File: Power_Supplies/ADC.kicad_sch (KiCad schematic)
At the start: 72 parts, among them IC1 PCM1808PWRG4, IC2 PCM1808PWRG4, IC3 PCM1808PWRG4, IC4 PCM1808PWRG4, IC5 PCM1808PWRG4, IC6 PCM1808PWRG4, IC7 PCM1808PWRG4, IC8 PCM1808PWRG4

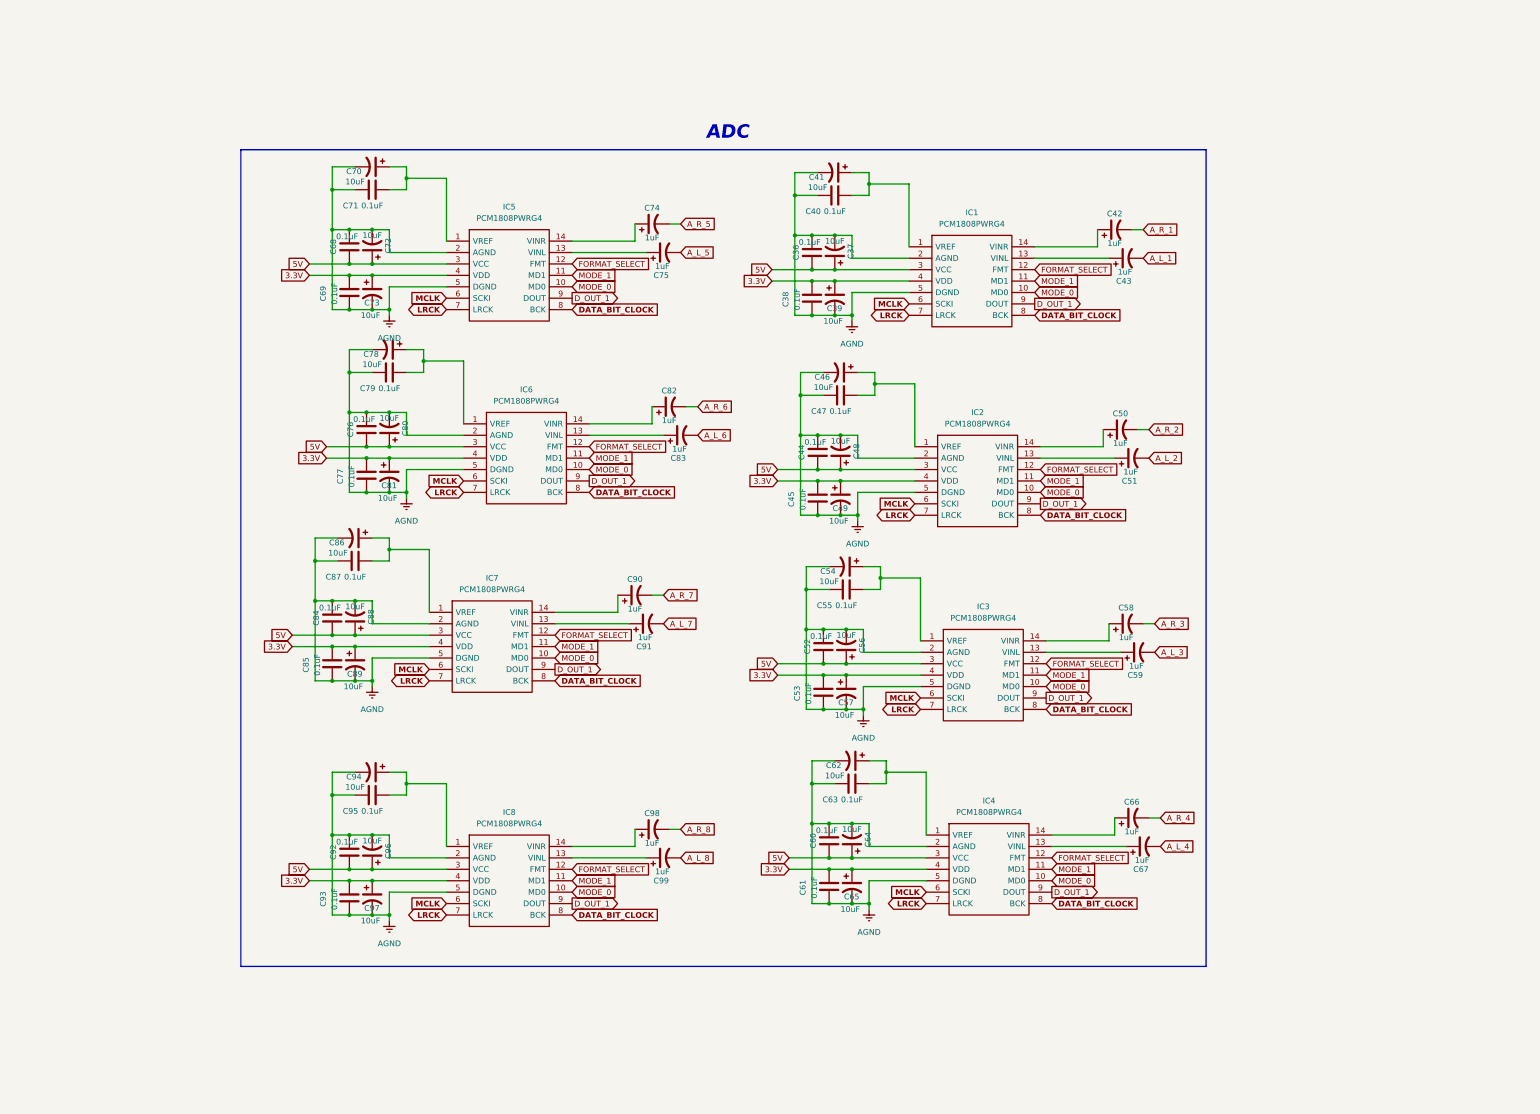
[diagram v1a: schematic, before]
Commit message: Add files via upload
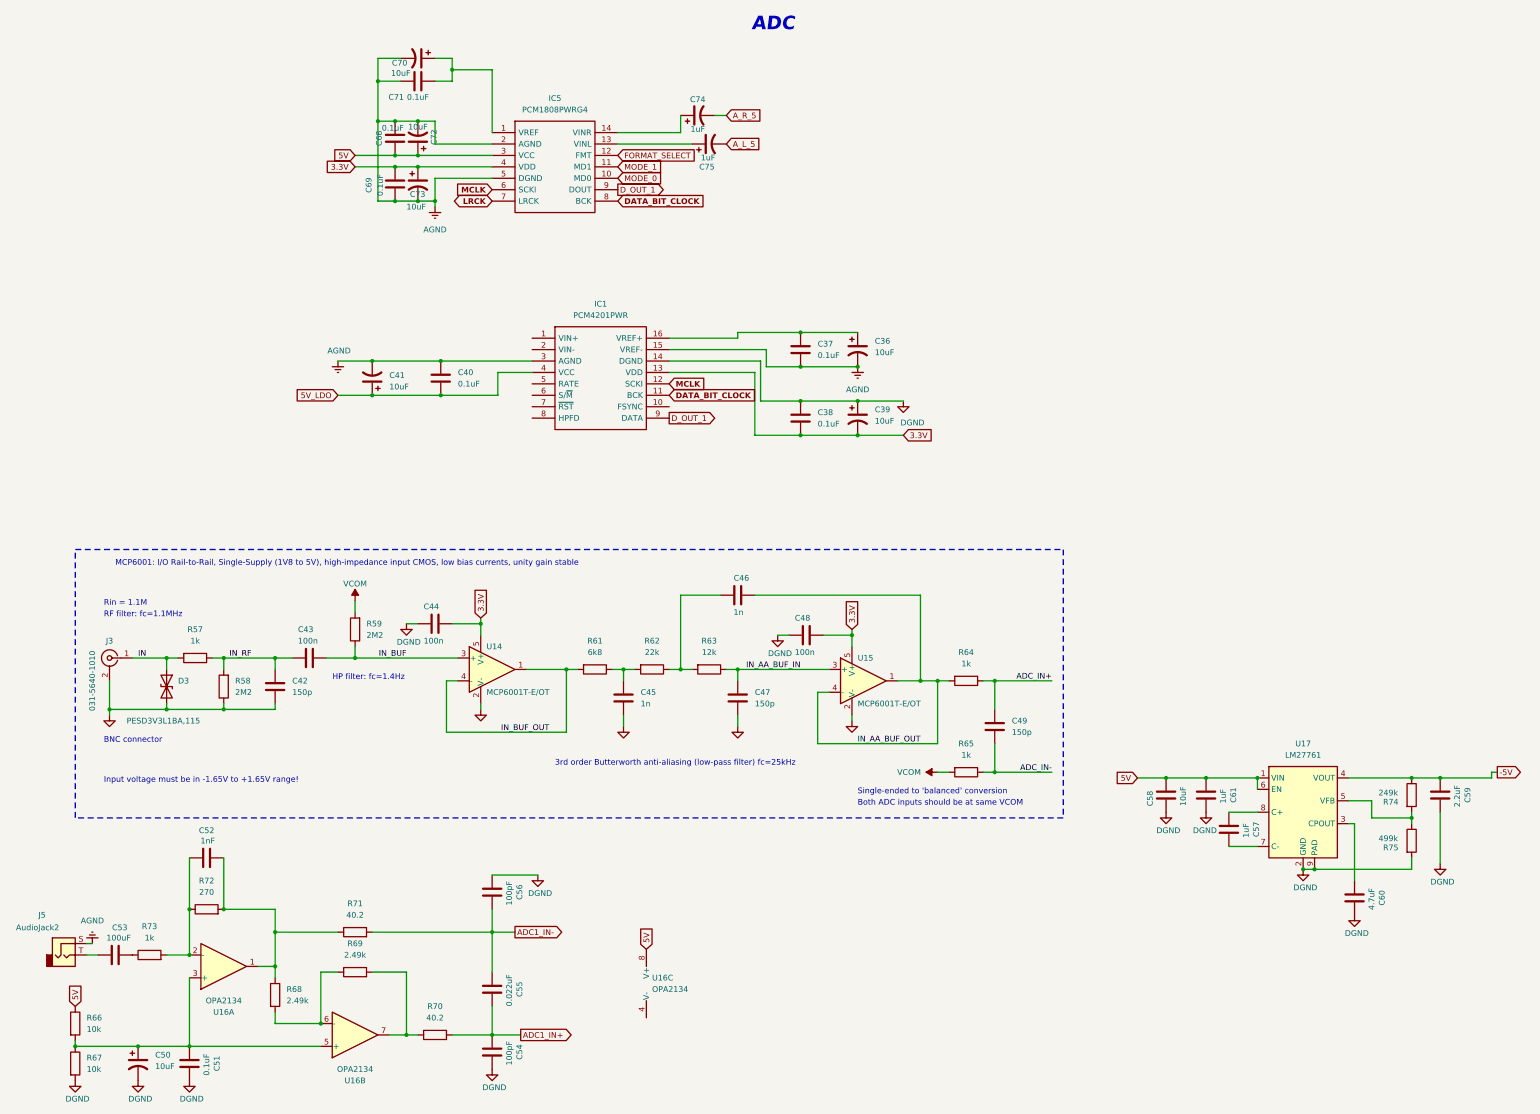
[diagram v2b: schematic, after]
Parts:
- removed C36, C63, C76, C77, C79, C84, C85, C87, C92, C93, C95: 0.1uF, Capacitor_SMD:C_0805_2012Metric, symbol Device:C
- removed C37, C46, C48, C49, C54, C56, C57, C62, C64, C65, C78, C80, C81, C86, C88, C89, C94, C96, C97: 10uF, Capacitor_SMD:CP_Elec_4x5.8, symbol Device:C_Polarized_US
- removed C42, C43, C51, C58, C59, C66, C67, C82, C83, C90, C91, C98, C99: 1uF, Capacitor_SMD:CP_Elec_4x5.8, symbol Device:C_Polarized_US
- removed IC1, IC2, IC3, IC4, IC6, IC7, IC8: PCM1808PWRG4, SamacSys_Parts:SOP65P640X120-14N, symbol SamacSys_Parts:PCM1808PWRG4
- added C36: 10uF, Capacitor_SMD:CP_Elec_4x5.8, symbol Device:C_Polarized_US
- added C37, C51: 0.1uF, Capacitor_SMD:C_0805_2012Metric, symbol Device:C
- added C42, C49: 150p, Capacitor_SMD:C_0402_1005Metric, symbol Device:C
- added C43, C48: 100n, Capacitor_SMD:C_0402_1005Metric, symbol Device:C
- added C46: 1n, Capacitor_SMD:C_0402_1005Metric, symbol Device:C
- added C54, C56: 100pF, Capacitor_SMD:C_0805_2012Metric, symbol Device:C
- added C57: 1uF, Capacitor_SMD:C_0805_2012Metric, symbol Device:C
- added C58: 10uF, Capacitor_SMD:C_0805_2012Metric, symbol Device:C
- added C59: 2.2uF, Capacitor_SMD:C_0805_2012Metric, symbol Device:C
- added D3: PESD3V3L1BA,115, Diode_SMD:D_SOD-323, symbol Device:D_TVS
- added IC1: PCM4201PWR, SOP65P640X120-16N, symbol SamacSys_Parts:PCM4201PWR
- added J3: 031-5640-1010, PhilsLab_Footprints_KiCad6:AMPHENOL-BNC-031-5640-1010, symbol Connector:Conn_Coaxial
- added J5: AudioJack2, symbol Connector_Audio:AudioJack2
- added R57, R64, R65: 1k, Resistor_SMD:R_0402_1005Metric, symbol Device:R
- added R58, R59: 2M2, Resistor_SMD:R_0402_1005Metric, symbol Device:R
- added R61: 6k8, Resistor_SMD:R_0402_1005Metric, symbol Device:R
- added R62: 22k, Resistor_SMD:R_0402_1005Metric, symbol Device:R
- added R63: 12k, Resistor_SMD:R_0402_1005Metric, symbol Device:R
- added R66, R67: 10k, Resistor_SMD:R_0805_2012Metric, symbol Device:R
- added R68, R69: 2.49k, Resistor_SMD:R_0805_2012Metric, symbol Device:R
- added R70, R71: 40.2, Resistor_SMD:R_0805_2012Metric, symbol Device:R
- added R72: 270, Resistor_SMD:R_0805_2012Metric, symbol Device:R
- added R73: 1k, Resistor_SMD:R_0805_2012Metric, symbol Device:R
- added R74: 249k, Resistor_SMD:R_0603_1608Metric, symbol Device:R
- added R75: 499k, Resistor_SMD:R_0603_1608Metric, symbol Device:R
- added U14, U15: MCP6001T-E/OT, Package_TO_SOT_SMD:SOT-23-5, symbol Amplifier_Operational:MCP6001-OT
- added U16: OPA2134, symbol Amplifier_Operational:OPA2134
- added U17: LM27761, Package_SON:WSON-8-1EP_2x2mm_P0.5mm_EP0.9x1.6mm, symbol Regulator_SwitchedCapacitor:LM27761
- C44: value 0.1uF -> 100n; footprint Capacitor_SMD:C_0805_2012Metric -> Capacitor_SMD:C_0402_1005Metric
- C45: value 0.1uF -> 1n; footprint Capacitor_SMD:C_0805_2012Metric -> Capacitor_SMD:C_0402_1005Metric
- C47: value 0.1uF -> 150p; footprint Capacitor_SMD:C_0805_2012Metric -> Capacitor_SMD:C_0402_1005Metric
- C50: value 1uF -> 10uF
- C52: value 0.1uF -> 1nF; footprint Capacitor_SMD:C_0805_2012Metric -> Capacitor_SMD:C_0402_1005Metric
- C53: value 0.1uF -> 100uF
- C55: value 0.1uF -> 0.022uF
- C60: value 0.1uF -> 4.7uF
- C61: value 0.1uF -> 1uF
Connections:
- net 3.3V: now also C39.2, C44.1, C48.1, IC1.13 (VDD), U14.5 (V+), U15.5 (V+); no longer C39.1, C45.2, C53.2, C61.2
- net 5V: now also C61.2, C58.2, R66.1, U16.8 (V+), U17.1 (VIN), U17.6 (EN); no longer C44.1, C52.1, C60.1
- net AGND: now also C40.1, C36.2, C37.2, IC1.15 (VREF-), IC1.3 (AGND), J5.S; no longer C38.1, C39.2, C40.2, C44.2, C45.1, C47.2, C52.2, C53.1, C55.2, C60.2, C61.1
- net DATA_BIT_CLOCK: now also IC1.11 (BCK)
- net D_OUT_1: now also IC1.9 (DATA)
- net MCLK: now also IC1.12 (SCKI)
- net ADC1_IN+: now reaches C55.1
- net ADC1_IN+: now also C54.2, R70.2
- net 5V_LDO: now reaches C41.1
- net 5V_LDO: now also C40.2, IC1.4 (VCC); no longer C40.1
- net IN_AA_BUF_IN: now reaches C47.1
- net IN_AA_BUF_IN: now also R63.1, U15.3 (+)
- net at C50.1: now also C51.2, R66.2, R67.1, U16.3 (+), U16.5 (+)
- net A_R_2 renamed DGND
- net DGND: now also C38.1, C39.1, C44.2, C60.1, C61.1, C48.2, C51.1, C54.1, C56.2, C58.1, C59.1, IC1.14 (DGND), R67.2, R75.2, U17.2 (GND), U17.9 (PAD)
- new net: C52.1, R68.1, R71.1, R72.2, U16.1
- new net: C52.2, R72.1, R73.2, U16.2 (-)
- new net: C46.1, R62.1, R63.2
- new net: C45.1, R61.1, R62.2
- new net: R68.2, R69.1, U16.6 (-)
- new net: C53.1, R73.1
- new net: C53.2, J5.T
- new net: R69.2, R70.1, U16.7
- new net: C36.1, C37.1, IC1.16 (VREF+)
- new net: R74.2, R75.1, U17.5 (VFB)
- new net: C60.2, U17.3 (CPOUT)
- new net: C57.1, U17.7 (C-)
- new net: C57.2, U17.8 (C+)
- new net -5V: C59.2, R74.1, U17.4 (VOUT)
- new net ADC1_IN-: C55.2, C56.1, R71.2
- new net ADC_IN+: C49.1, R64.1
- new net ADC_IN-: C49.2, R65.1
- new net GND: C42.2, C45.2, C47.2, D3.2 (A2), J3.2 (Ext), R58.1, U14.2 (V-), U15.2 (V-)
- new net IN: D3.1 (A1), J3.1 (In), R57.2
- new net IN_AA_BUF_OUT: C46.2, R64.2, U15.1, U15.4 (-)
- new net IN_BUF: C43.1, R59.1, U14.3 (+)
- new net IN_BUF_OUT: R61.2, U14.1, U14.4 (-)
- new net IN_RF: C42.1, C43.2, R57.1, R58.2
- new net VCOM: R59.2, R65.2
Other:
- note added: "3rd order Butterworth anti-aliasing (low-pass filter) fc=25kHz"
- note added: "BNC connector"
- note added: "Both ADC inputs should be at same VCOM"
- note added: "HP filter: fc=1.4Hz"
- note added: "Input voltage must be in -1.65V to +1.65V range!"
- note added: "MCP6001: I/O Rail-to-Rail, Single-Supply (1V8 to 5V), high-impedance input CMOS, low bias currents, unity gain stable"
- note added: "RF filter: fc=1.1MHz"
- note added: "Rin = 1.1M"
- note added: "Single-ended to 'balanced' conversion"
- moved on the sheet: C68, C69, C70, C71, C72, C73, C74, C75, IC5

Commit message: Add files via upload
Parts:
- removed C42, C47, C49: 150p, Capacitor_SMD:C_0402_1005Metric, symbol Device:C
- removed C43, C44, C48: 100n, Capacitor_SMD:C_0402_1005Metric, symbol Device:C
- removed C45, C46: 1n, Capacitor_SMD:C_0402_1005Metric, symbol Device:C
- removed C50, C70, C72, C73: 10uF, Capacitor_SMD:CP_Elec_4x5.8, symbol Device:C_Polarized_US
- removed C51, C68: 0.1uF, Capacitor_SMD:C_0805_2012Metric, symbol Device:C
- removed C74: 1uF, Capacitor_SMD:CP_Elec_4x5.8, symbol Device:C_Polarized_US
- removed D3: PESD3V3L1BA,115, Diode_SMD:D_SOD-323, symbol Device:D_TVS
- removed IC5: PCM1808PWRG4, SamacSys_Parts:SOP65P640X120-14N, symbol SamacSys_Parts:PCM1808PWRG4
- removed J3: 031-5640-1010, PhilsLab_Footprints_KiCad6:AMPHENOL-BNC-031-5640-1010, symbol Connector:Conn_Coaxial
- removed U14, U15: MCP6001T-E/OT, Package_TO_SOT_SMD:SOT-23-5, symbol Amplifier_Operational:MCP6001-OT
- added C121, C122, C123, C124, C70, C77, C84: 1nF, Capacitor_SMD:C_0402_1005Metric, symbol Device:C
- added C125, C127, C128, C130, C131, C133, C134, C136, C73, C78, C80, C85, C87: 100pF, Capacitor_SMD:C_0805_2012Metric, symbol Device:C
- added C126, C129, C132, C135, C72, C79, C86: 0.022uF, Capacitor_SMD:C_0805_2012Metric, symbol Device:C
- added C50, C67, C74, C81, C88, C89, C90, C91: 100uF, Capacitor_SMD:C_0805_2012Metric, symbol Device:C
- added C51, C68, C82, C92, C93, C94, C95: 10uF, Capacitor_SMD:CP_Elec_4x5.8, symbol Device:C_Polarized_US
- added C62: 10uF, Capacitor_SMD:C_0805_2012Metric, symbol Device:C
- added C63, C64: 1uF, Capacitor_SMD:C_0805_2012Metric, symbol Device:C
- added C65: 4.7uF, Capacitor_SMD:C_0805_2012Metric, symbol Device:C
- added C66: 2.2uF, Capacitor_SMD:C_0805_2012Metric, symbol Device:C
- added C76, C83, C96, C97, C98, C99: 0.1uF, Capacitor_SMD:C_0805_2012Metric, symbol Device:C
- added J10, J11, J12, J13, J3, J7, J9: AudioJack2, symbol Connector_Audio:AudioJack2
- added R100, R101, R78, R79, R86, R87, R94, R95, R96, R97, R98, R99: 10k, Resistor_SMD:R_0805_2012Metric, symbol Device:R
- added R102, R103, R104, R105, R80, R88: 1k, Resistor_SMD:R_0805_2012Metric, symbol Device:R
- added R106, R107, R108, R109, R81, R89: 270, Resistor_SMD:R_0805_2012Metric, symbol Device:R
- added R110, R111, R112, R113, R115, R117, R119, R121, R82, R84, R90, R92: 2.49k, Resistor_SMD:R_0805_2012Metric, symbol Device:R
- added R114, R116, R118, R120, R122, R123, R124, R125, R83, R85, R91, R93: 40.2, Resistor_SMD:R_0805_2012Metric, symbol Device:R
- added R76: 249k, Resistor_SMD:R_0603_1608Metric, symbol Device:R
- added R77: 499k, Resistor_SMD:R_0603_1608Metric, symbol Device:R
- added U14, U15, U19, U20, U21, U22, U23: OPA2134, symbol Amplifier_Operational:OPA2134
- added U18: LM27761, Package_SON:WSON-8-1EP_2x2mm_P0.5mm_EP0.9x1.6mm, symbol Regulator_SwitchedCapacitor:LM27761
- C52: value 1nF -> 0.1uF; footprint Capacitor_SMD:C_0402_1005Metric -> Capacitor_SMD:C_0805_2012Metric
- C53: value 100uF -> 1nF; footprint Capacitor_SMD:C_0805_2012Metric -> Capacitor_SMD:C_0402_1005Metric
- C71: value 0.1uF -> 100pF
- C75: value 1uF -> 10uF
- R57: value 1k -> 10k; footprint Resistor_SMD:R_0402_1005Metric -> Resistor_SMD:R_0805_2012Metric
- R58: value 2M2 -> 10k; footprint Resistor_SMD:R_0402_1005Metric -> Resistor_SMD:R_0805_2012Metric
- R59: value 2M2 -> 1k; footprint Resistor_SMD:R_0402_1005Metric -> Resistor_SMD:R_0805_2012Metric
- R61: value 6k8 -> 270; footprint Resistor_SMD:R_0402_1005Metric -> Resistor_SMD:R_0805_2012Metric
- R62: value 22k -> 2.49k; footprint Resistor_SMD:R_0402_1005Metric -> Resistor_SMD:R_0805_2012Metric
- R63: value 12k -> 40.2; footprint Resistor_SMD:R_0402_1005Metric -> Resistor_SMD:R_0805_2012Metric
- R64: value 1k -> 2.49k; footprint Resistor_SMD:R_0402_1005Metric -> Resistor_SMD:R_0805_2012Metric
- R65: value 1k -> 40.2; footprint Resistor_SMD:R_0402_1005Metric -> Resistor_SMD:R_0805_2012Metric
- R68: value 2.49k -> 1k
- R69: value 2.49k -> 270
- R70: value 40.2 -> 2.49k
- R72: value 270 -> 2.49k
- R73: value 1k -> 40.2
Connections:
- net -5V is gone; now on net -5V_1: C59.2, R74.1, U17.4 (VOUT)
- net A_L_5 is gone; now on net DGND: C75.2
- net IN is gone; now on an unnamed net: R57.2
- net IN_AA_BUF_IN is gone; now on an unnamed net: R63.1
- net IN_AA_BUF_OUT is gone; now on an unnamed net: R64.2
- net IN_BUF_OUT is gone; now on an unnamed net: R61.2
- net 3.3V: no longer C69.2
- net 5V: now also R57.1, C62.2, C63.2, R100.1, R78.1, R86.1, R94.1, R96.1, R98.1, U14.8 (V+), U15.8 (V+), U18.1 (VIN), U18.6 (EN), U19.8 (V+), U20.8 (V+), U21.8 (V+), U22.8 (V+), U23.8 (V+)
- net ADC1_IN+: now also C56.2, IC1.1 (VIN+), R65.2; no longer C54.2, R70.2
- net ADC1_IN-: now also C54.1, IC1.2 (VIN-), R63.2; no longer C56.1, R71.2
- net AGND: now also J10.S, J11.S, J12.S, J13.S, J3.S, J7.S, J9.S; no longer C69.1, C71.2
- net DGND: now also C52.1, C54.2, C56.1, C69.1, C71.2, R58.2, C125.2, C127.1, C128.2, C130.1, C131.2, C133.1, C134.2, C136.1, C51.2, C62.1, C63.1, C65.1, C66.1, C68.2, C73.1, C76.1, C78.2, C80.1, C82.2, C83.1, C85.2, C87.1, C92.2, C93.2, C94.2, C95.2, C96.1, C97.1, C98.1, C99.1, R101.2, R77.2, R79.2, R87.2, R95.2, R97.2, R99.2, U18.2 (GND), U18.9 (PAD); no longer C54.1, C56.2
- net at U16.3 (+), U16.5 (+): now also C75.1, C76.2, R78.2, R79.1; no longer R66.2, R67.1
- net at R62.1: now also C53.1, U14.1; no longer R63.2
- net at R61.1: now also C53.2, R59.2, U14.2 (-); no longer R62.2
- net at R68.2, R69.1: now also C70.2, U15.2 (-); no longer U16.6 (-)
- net at R73.1: now also R72.2, U15.7; no longer C53.1
- net at J5.T: now also C67.2; no longer C53.2
- net at R69.2, R70.1: now also R71.1, C70.1, U15.1; no longer U16.7
- net ADC2_IN-: now reaches C71.1
- net ADC2_IN-: now also R71.2, C72.2, C78.1, C79.2, C85.1, C86.2, R83.2, R91.2
- net -5V_1: now reaches U16.4 (V-)
- net -5V_1: now also U14.4 (V-), U15.4 (V-), U19.4 (V-)
- net ADC_IN+: no longer names the net of R64.1
- net ADC_IN+: now also R62.2, U14.6 (-)
- net ADC_IN-: no longer names the net of R65.1
- net ADC_IN-: now also U14.7
- net GND: no longer names the net of R58.1
- net GND: now also C52.2, C51.1, U14.3 (+), U14.5 (+)
- net IN_BUF: no longer names the net of R59.1
- net IN_BUF: now also C50.1
- removed net IN_RF: R57.1, R58.2
- removed net VCOM: R59.2, R65.2
- new net: C93.1, C97.2, R96.2, R97.1, U21.3 (+), U21.5 (+)
- new net: C122.1, R107.2, R111.1, R116.1, U21.1
- new net: C122.2, R103.2, R107.1, U21.2 (-)
- new net: R111.2, R117.1, U21.6 (-)
- new net: R117.2, R123.1, U21.7
- new net: R76.2, R77.1, U18.5 (VFB)
- new net: C77.1, R81.2, R82.1, R83.1, U16.1
- new net: C77.2, R80.2, R81.1, U16.2 (-)
- new net: C68.1, C69.2, R66.2, R67.1, U15.3 (+), U15.5 (+)
- new net: C123.1, R108.2, R112.1, R118.1, U22.1
- new net: R112.2, R119.1, U22.6 (-)
- new net: C91.1, R105.1
- new net: C124.2, R105.2, R109.1, U23.2 (-)
- new net: C89.2, J11.T
- new net: C64.1, U18.7 (C-)
- new net: C64.2, U18.8 (C+)
- new net: C95.1, C99.2, R100.2, R101.1, U23.3 (+), U23.5 (+)
- new net: C121.1, R106.2, R110.1, R114.1, U20.1
- new net: R110.2, R115.1, U20.6 (-)
- new net: C50.2, J3.T
- new net: R90.2, R92.1, U19.6 (-)
- new net: R92.2, R93.1, U19.7
- new net: C124.1, R109.2, R113.1, R120.1, U23.1
- new net: R70.2, R72.1, U15.6 (-)
- new net: C88.2, J10.T
- new net: C90.2, J12.T
- new net: C89.1, R103.1
- new net: C82.1, C83.2, R86.2, R87.1, U19.3 (+), U19.5 (+)
- new net: C88.1, R102.1
- new net: C81.1, R88.1
- new net: C84.2, R88.2, R89.1, U19.2 (-)
- new net: C94.1, C98.2, R98.2, R99.1, U22.3 (+), U22.5 (+)
- new net: R119.2, R124.1, U22.7
- new net: C84.1, R89.2, R90.1, R91.1, U19.1
- new net: C65.2, U18.3 (CPOUT)
- new net: C91.2, J13.T
- new net: C81.2, J9.T
- new net: C121.2, R102.2, R106.1, U20.2 (-)
- new net: R113.2, R121.1, U23.6 (-)
- new net: R121.2, R125.1, U23.7
- new net: C90.1, R104.1
- new net: C123.2, R104.2, R108.1, U22.2 (-)
- new net: R115.2, R122.1, U20.7
- new net: C92.1, C96.2, R94.2, R95.1, U20.3 (+), U20.5 (+)
- new net: R82.2, R84.1, U16.6 (-)
- new net: R84.2, R85.1, U16.7
- new net: C67.1, R68.1
- new net: C74.1, R80.1
- new net: C74.2, J7.T
- new net -5V_2: C66.2, R76.1, U18.4 (VOUT), U20.4 (V-), U21.4 (V-), U22.4 (V-), U23.4 (V-)
- new net ADC2_IN+: C72.1, C73.2, C79.1, C80.2, C86.1, C87.2, R73.2, R85.2, R93.2
- new net ADC5_IN+: C132.1, C133.2, R124.2
- new net ADC5_IN-: C131.1, C132.2, R118.2
- new net ADC6_IN+: C135.1, C136.2, R125.2
- new net ADC6_IN-: C134.1, C135.2, R120.2
- new net ADC7_IN+: C126.1, C127.2, R122.2
- new net ADC7_IN-: C125.1, C126.2, R114.2
- new net ADC8_IN+: C129.1, C130.2, R123.2
- new net ADC8_IN-: C128.1, C129.2, R116.2
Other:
- note added: "4 of the LM27761's go to the first inverter, the other 4 go to the second one."
- note added: "Buffers for each ADC's Inputs"
- note added: "Voltage Inverter w/ Max current output of 250mA Each OPA2134 uses 38mA max current, meaning for the 9 being used with dual supplies we need 2 LM27761s."
- note added: "Voltage Inverters for OPA2134's"
- note removed: "3rd order Butterworth anti-aliasing (low-pass filter) fc=25kHz"
- note removed: "ADC"
- note removed: "BNC connector"
- note removed: "Both ADC inputs should be at same VCOM"
- note removed: "HP filter: fc=1.4Hz"
- note removed: "Input voltage must be in -1.65V to +1.65V range!"
- note removed: "MCP6001: I/O Rail-to-Rail, Single-Supply (1V8 to 5V), high-impedance input CMOS, low bias currents, unity gain stable"
- note removed: "RF filter: fc=1.1MHz"
- note removed: "Rin = 1.1M"
- note removed: "Single-ended to 'balanced' conversion"
- moved on the sheet: C36, C37, C38, C39, C40, C41, C57, C58, C59, C60, C61, IC1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
